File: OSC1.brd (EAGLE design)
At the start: 27.6 x 54 mm, 23 parts

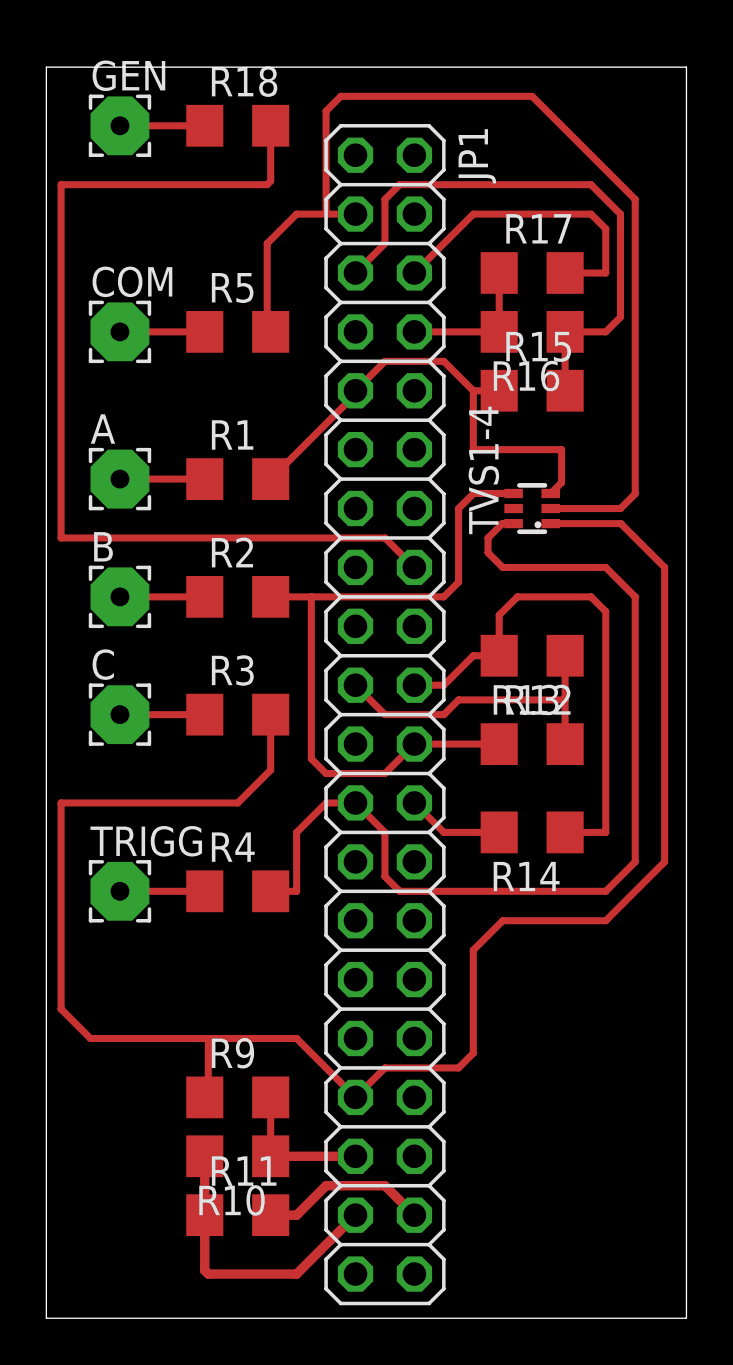
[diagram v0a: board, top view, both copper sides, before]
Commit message: Board retraced
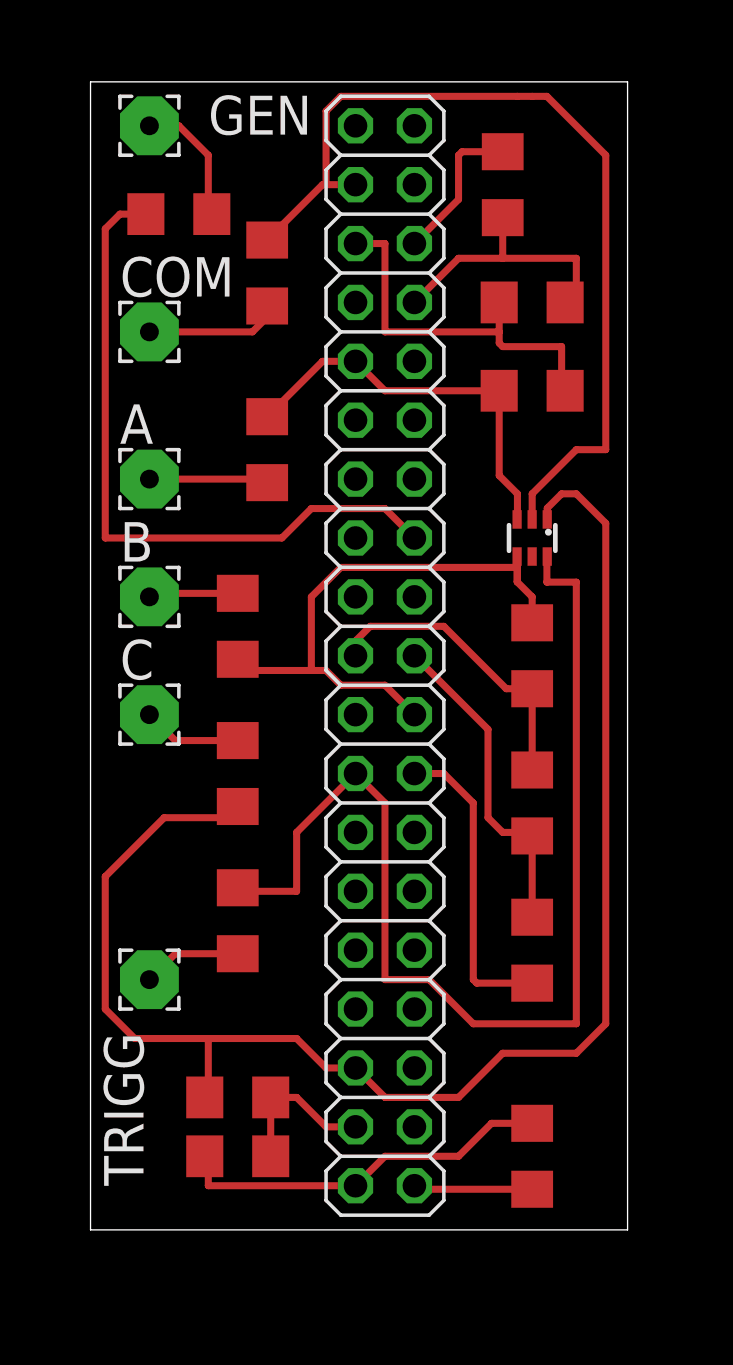
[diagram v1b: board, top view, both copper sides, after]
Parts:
- JP1: value STM32F3DISCO-LEFT -> STM32F3-DISCO LEFT; device pinhead:2X20 -> pinhead:2X19
- moved R11 13.0 mm to (21.0, 6.99), turned to 270 degrees
- moved R13 6.35 mm to (21.0, 22.2), turned to 270 degrees
- moved R14 5.08 mm to (21.0, 15.9), turned to 270 degrees
- moved R18 4.58 mm to (5.71, 47.6), turned to 180 degrees
- moved R17 4.02 mm to (19.7, 48.9), turned to 90 degrees
- moved TRIGG 4.02 mm to (4.45, 14.6)
- moved R12 3.81 mm to (21.0, 28.6), turned to 270 degrees
- moved R5 2.84 mm to (9.53, 45.1), turned to 90 degrees
- moved JP1 2.54 mm to (14.6, 28.6)
- moved R3 2.54 mm to (8.26, 23.5), turned to 270 degrees
- moved R1 1.80 mm to (9.53, 37.5), turned to 90 degrees
- moved A 1.27 mm to (4.45, 36.2)
- moved B 1.27 mm to (4.45, 31.1)
- moved C 1.27 mm to (4.45, 26.0)
- moved COM 1.27 mm to (4.45, 42.5)
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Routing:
- net DAC: track 42.5 -> 29.7 mm
- net C1: track 76.4 -> 65.2 mm
- net B2: track 4.18 -> 13.3 mm
- net B10: track 22.4 -> 14.0 mm
- net A30: track 24.3 -> 16.5 mm
- net A2: track 13.2 -> 6.57 mm
- net EXT_TRG: track 42.7 -> 48.6 mm
- net GND: track 44.7 -> 39.1 mm
- net A10: track 6.20 -> 11.6 mm
- net B1: track 30.1 -> 25.0 mm
- net C10: track 12.5 -> 16.4 mm
- net A1: track 21.0 -> 17.4 mm
- net N$1: track 3.66 -> 5.83 mm
- net C2: track 7.25 -> 5.14 mm
- net N$19: track 3.66 -> 5.67 mm
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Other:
- board size 27.6 x 54 mm -> 23.2 x 49.5 mm
- board text added: "STM32F3-DISCOVERY OSCILLOSCOPE"
- board text added: "TOP LEFT->"
- board text added: "TOP-> LFT->"
- board text added: "https://goo.gl/CjWM7u"
